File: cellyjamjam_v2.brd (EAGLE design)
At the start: 107.4 x 82.6 mm, 42 parts, among them IC4 LM1458, Q2 MMBT3904

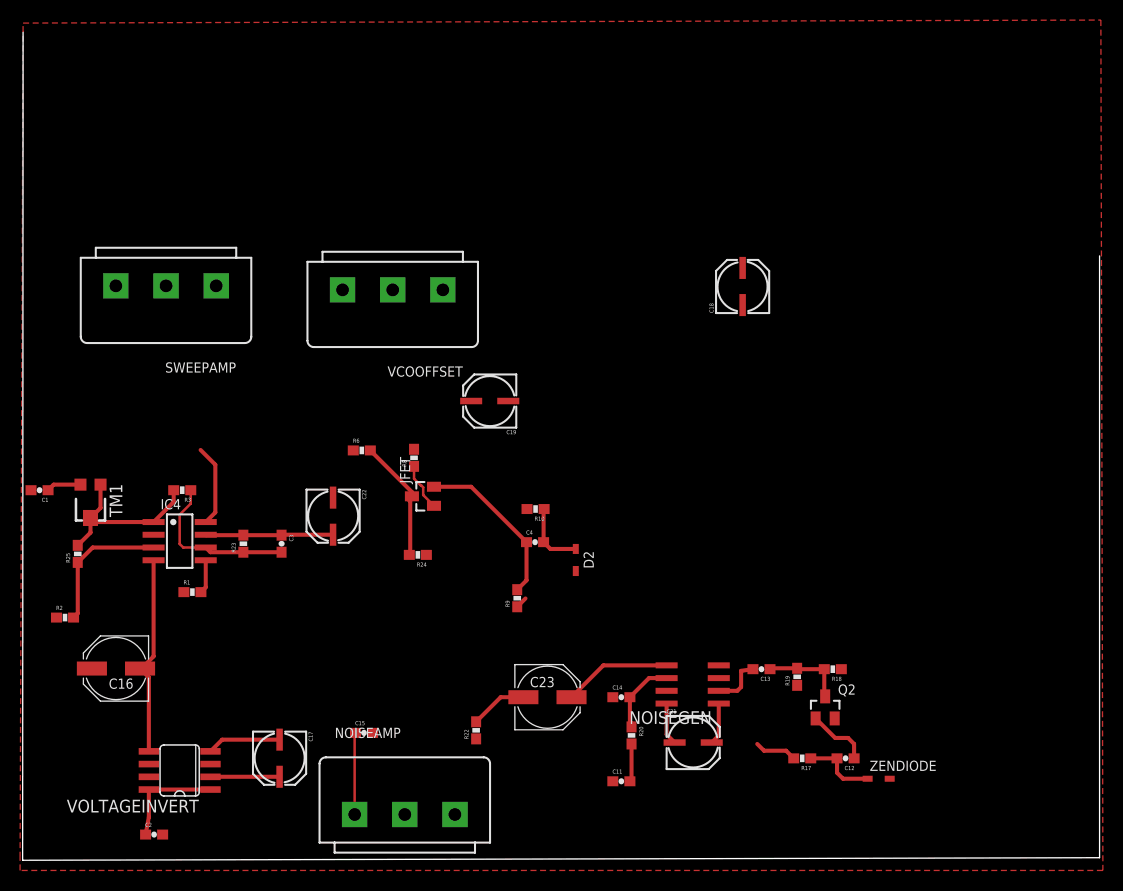
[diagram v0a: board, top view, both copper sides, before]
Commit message: designin'
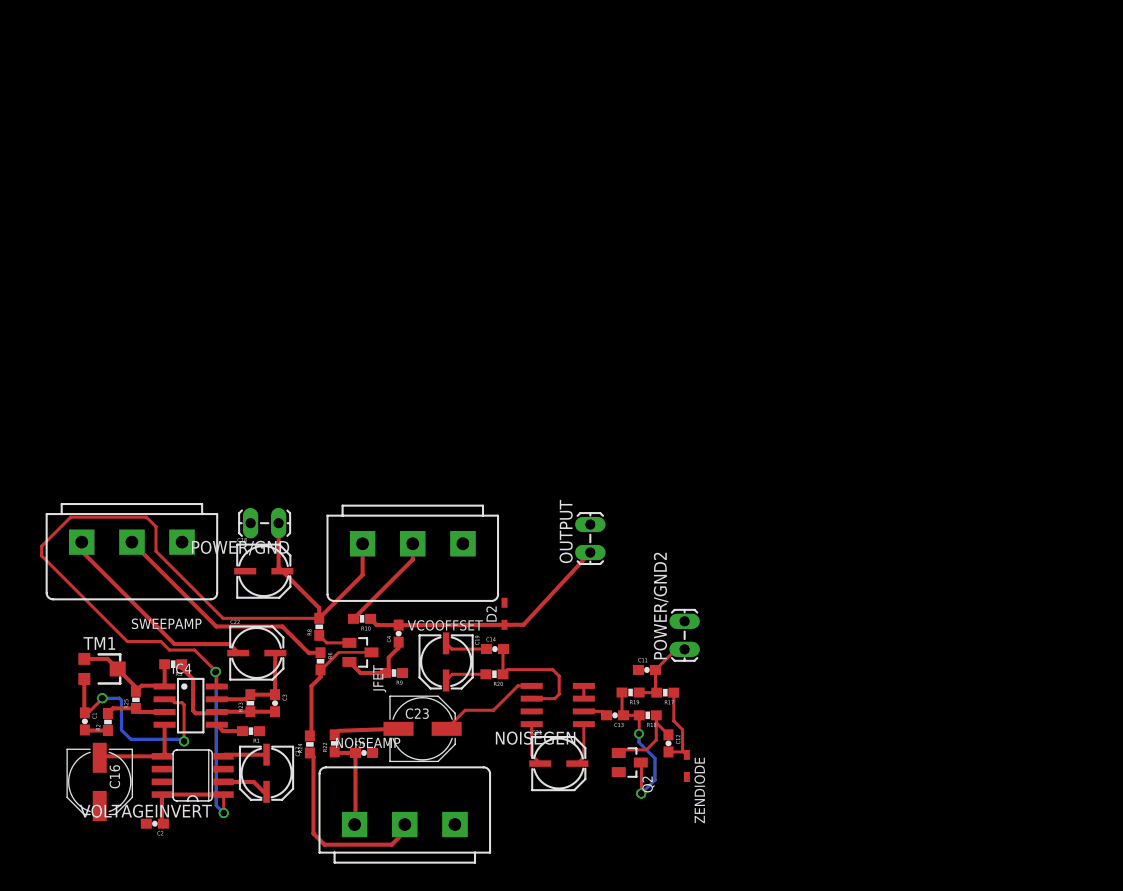
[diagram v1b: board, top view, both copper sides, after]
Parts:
- added OUTPUT: out, SparkFun-Connectors:1X02_LOCK_LONGPADS
- added POWER/GND, POWER/GND2: (no value), SparkFun-Connectors:1X02_LOCK_LONGPADS
- NOISEAMP, SWEEPAMP: value 5K/10TURN -> 5K
- VCOOFFSET: value 5K/10TURN -> 5k
- moved C18 55.3 mm to (24.2, 28.8), turned to 0 degrees
- moved C19 26.1 mm to (42.7, 19.6), turned to 270 degrees
- moved SWEEPAMP 25.8 mm to (11.2, 35.3)
- moved VCOOFFSET 25.4 mm to (39.1, 35.1)
- moved C1 23.5 mm to (6.46, 13.6), turned to 270 degrees
- moved R24 21.7 mm to (28.9, 11.3), turned to 90 degrees
- moved R6 21.4 mm to (30.0, 19.6), turned to 270 degrees
- moved R10 20.5 mm to (34.1, 23.8)
- moved Q2 20.2 mm to (60.8, 9.49), turned to 270 degrees
- moved R8 19.3 mm to (29.8, 23.0)
- moved ZENDIODE 19.2 mm to (66.5, 9.15), turned to 270 degrees
- moved R18 19.0 mm to (62.6, 14.2)
- moved C12 17.7 mm to (64.6, 11.4), turned to 270 degrees
- moved R3 17.4 mm to (15.3, 19.3)
- moved JFET 16.8 mm to (33.9, 20.5), turned to 270 degrees
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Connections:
- new net N$33: C11.2, POWER/GND2.1, R17.2, R19.1
- net GND: now also OUTPUT.2, POWER/GND.2, POWER/GND2.2, VCOOFFSET.1; no longer VCOOFFSET.3
- net N$52: now also OUTPUT.1
- net VCC: now also POWER/GND.1, VCOOFFSET.3; no longer C11.2, R17.2, R19.1, VCOOFFSET.1
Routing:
- net VCC: track 27.1 -> 109.4 mm, vias 0 -> 2
- net N$11: track 0.00 -> 23.4 mm
- net N$12: track 0.00 -> 20.7 mm
- net N$10: track 3.46 -> 23.2 mm, vias 0 -> 2
- net N$25: track 0.00 -> 19.0 mm
- net N$52: track 6.82 -> 25.3 mm
- net N$7: track 19.9 -> 9.52 mm
- net N$31: track 0.00 -> 9.94 mm
- net N$30: track 16.6 -> 7.67 mm
- net N$33: track 0.00 -> 7.84 mm
- net N$49: track 13.8 -> 6.01 mm
- net N$19: track 8.23 -> 16.0 mm, vias 0 -> 2
- net GND: track 1.23 -> 7.85 mm
- net N$26: track 7.48 -> 13.3 mm
- net N$8: track 17.5 -> 12.1 mm
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- removed copper zone on layer 1, net GND
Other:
- board outline removed

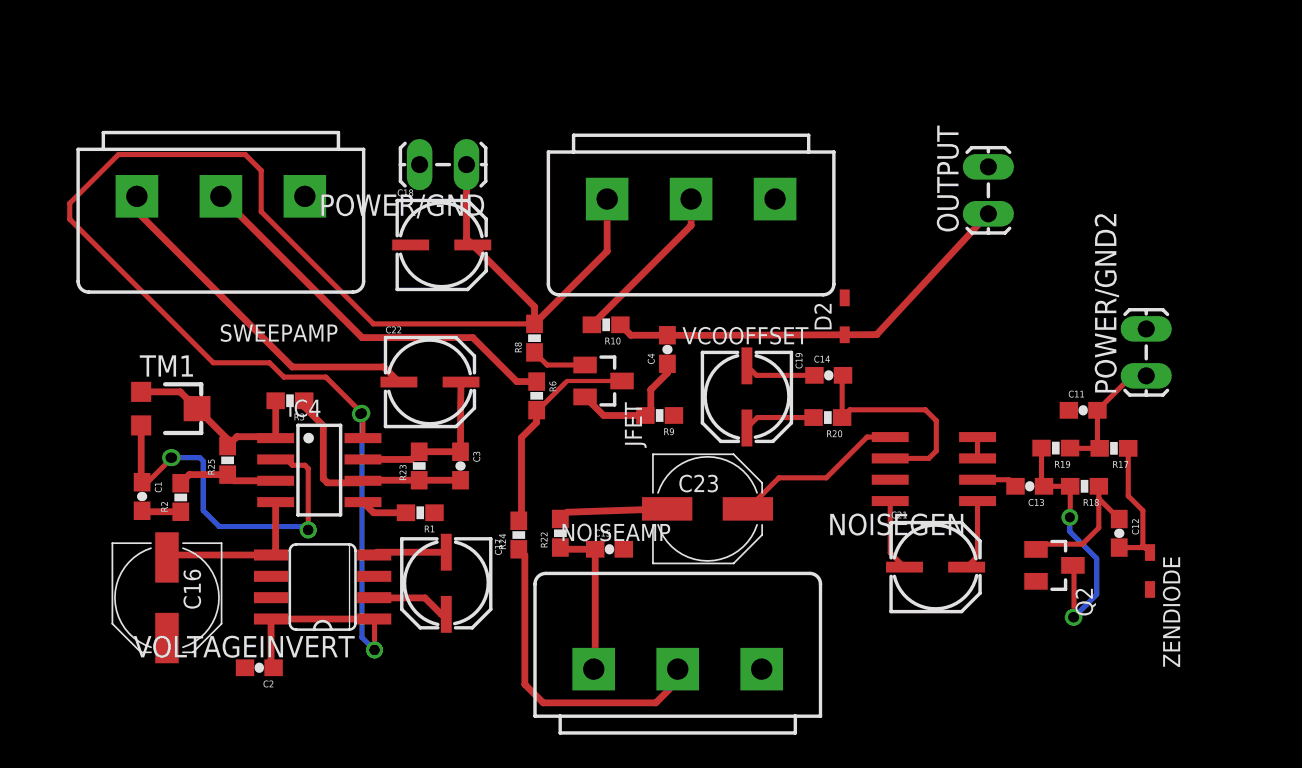
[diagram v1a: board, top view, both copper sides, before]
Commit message: fuuuuuuu had to hand draw the ulp
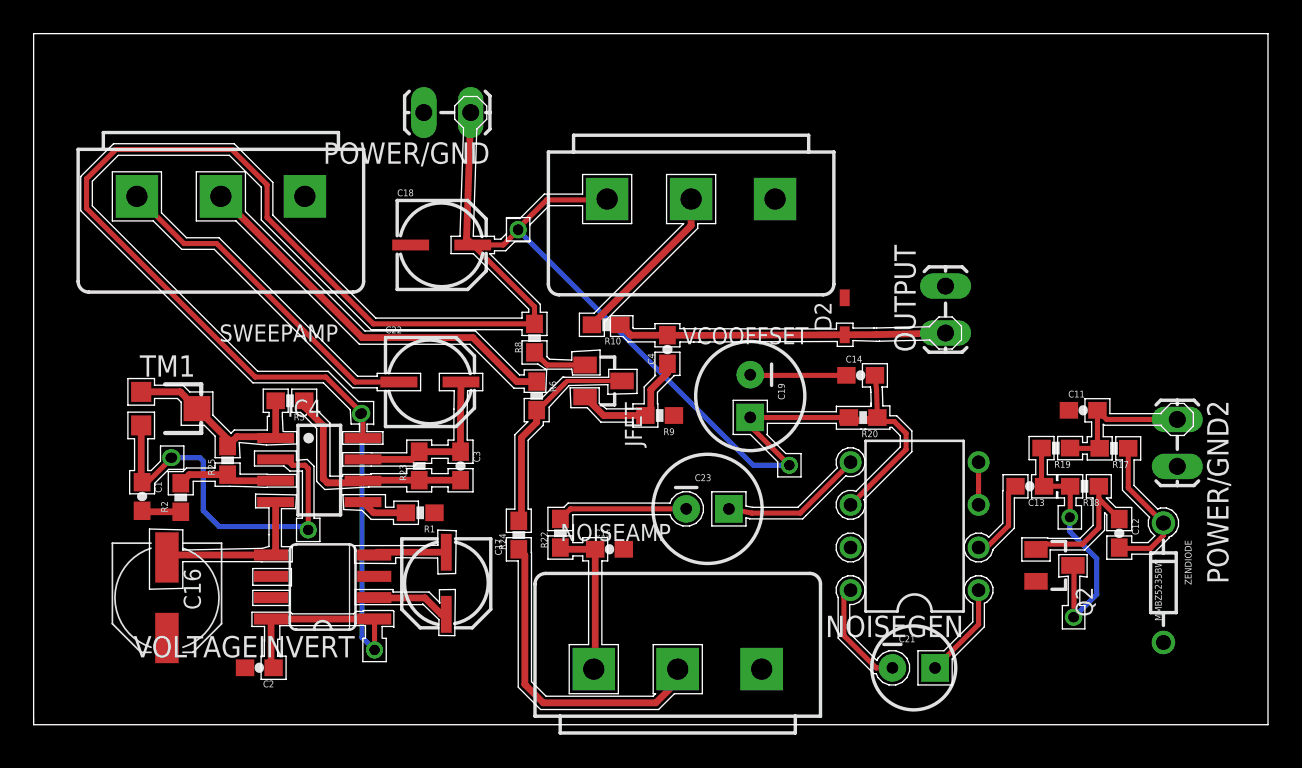
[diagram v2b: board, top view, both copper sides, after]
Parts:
- C19: device SparkFun-Capacitors:PANASONIC_C -> SparkFun-Capacitors:CPOL-RADIAL-100UF-25V
- C21: device SparkFun-Capacitors:PANASONIC_C -> SparkFun-Capacitors:CPOL-RADIAL-10UF-25V
- C23: device SparkFun-Capacitors:PANASONIC_D -> SparkFun-Capacitors:CPOL-RADIAL-100UF-25V
- IC4: device linear:SO08 -> linear:SO08@2
- NOISEGEN: value LM386M-1 -> LM386N-1; device linear:SO08@1 -> linear:DIL08
- ZENDIODE: device zetex:SOD323 -> SparkFun-DiscreteSemi:DIODE-ZENER
- moved OUTPUT 7.54 mm to (54.3, 23.4)
- moved C21 6.32 mm to (52.4, 3.38)
- moved NOISEGEN 3.59 mm to (52.5, 11.8)
- moved POWER/GND2 3.40 mm to (68.1, 18.1), turned to 270 degrees
- moved POWER/GND 3.11 mm to (25.9, 36.5)
- moved R20 2.10 mm to (49.4, 18.3)
- moved C14 1.90 mm to (49.2, 20.8)
- moved ZENDIODE 1.06 mm to (67.3, 8.45)
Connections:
- net GND: now also C19.2, ZENDIODE.P$2; no longer C19.-, ZENDIODE.2
- net N$15: now also C21.2; no longer C21.-
- net N$20: now also ZENDIODE.P$1; no longer ZENDIODE.1
- net N$21: now also C23.2; no longer C23.-
- net N$22: now also C23.1; no longer C23.+
- net N$6: now also C21.1; no longer C21.+
- net VCC: now also C19.1; no longer C19.+
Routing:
- net VCC: track 109.4 -> 138.3 mm, vias 2 -> 4
- net N$52: track 25.3 -> 19.6 mm
- net GND: track 7.85 -> 10.6 mm
- net N$18: track 2.42 -> 4.84 mm
- net N$15: track 4.29 -> 6.56 mm
- net N$22: track 10.2 -> 8.55 mm
- net N$6: track 4.20 -> 5.70 mm
- net N$33: track 7.84 -> 9.07 mm
- net N$21: track 6.53 -> 7.74 mm
- net N$26: track 13.3 -> 14.5 mm
- net N$12: track 20.7 -> 20.2 mm
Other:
- board outline added: 73.5 x 41.1 mm
